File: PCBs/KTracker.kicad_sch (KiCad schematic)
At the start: 63 parts, among them J1 Conn_01x02_Female, J2 Conn_01x04_Female, J3 Conn_01x02_Female, J4 Conn_01x08_Female, J5 Conn_01x02_Female, P1 USB_C_Plug_USB2.0, SW1 Option/FLASH Switch, SW2 Cali Switch, SW3 SW_SPDT MAIN POWER, U1 ME6211C, U2 TP4056, U3 MPU-6050, U4 DW01, U5 FS8205A, U6 ESP-12F, U7 CH340C, U8 QMC5883L

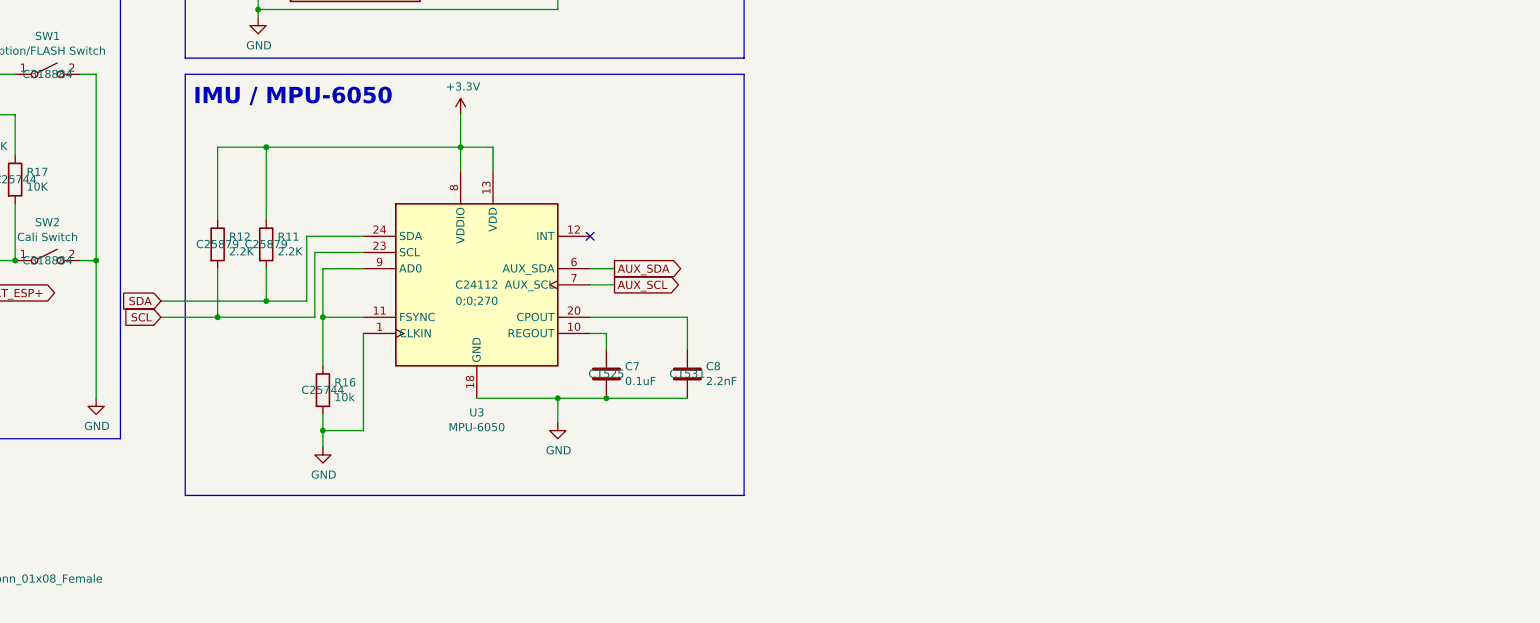
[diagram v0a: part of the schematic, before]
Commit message: #auto_saved_files#
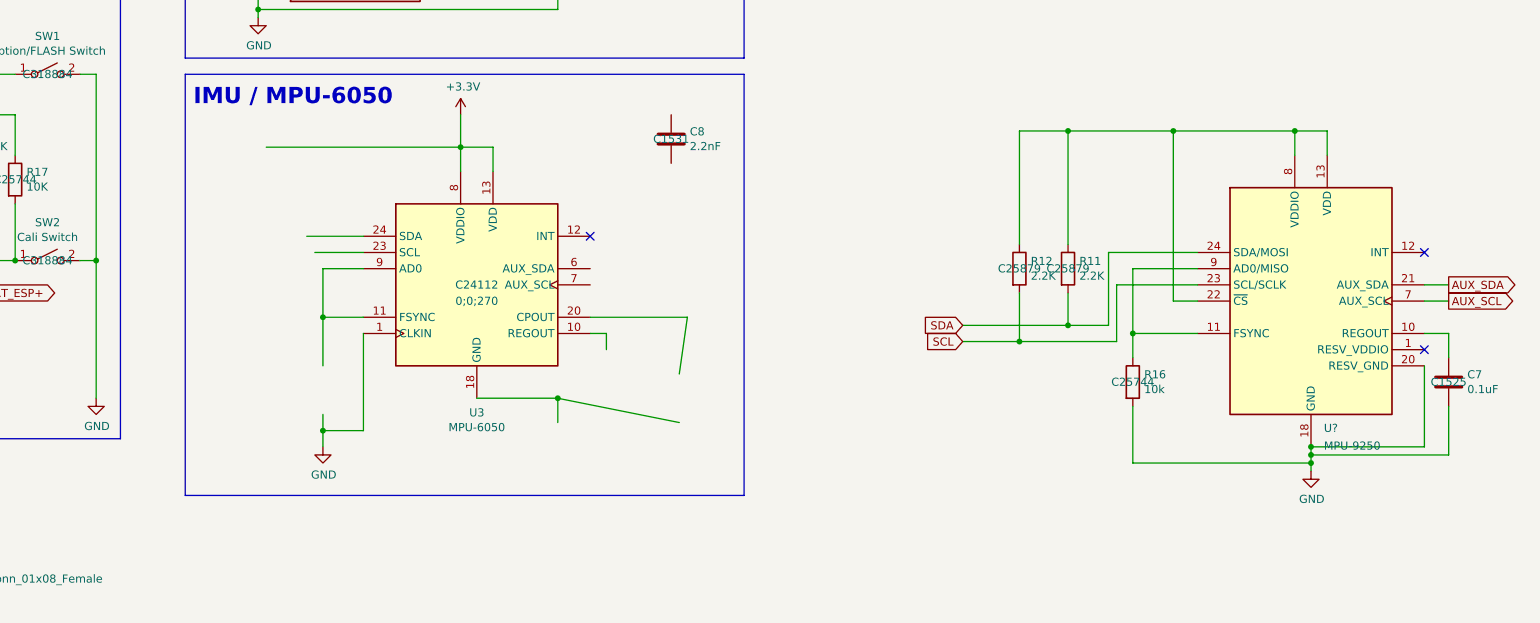
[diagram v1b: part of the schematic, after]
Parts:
- added U?: MPU-9250, Sensor_Motion:InvenSense_QFN-24_3x3mm_P0.4mm, symbol Sensor_Motion:MPU-9250
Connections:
- net +3V3: no longer R11.1, R12.1
- net AUX_SCL: now also U?.7 (AUX_SCL); no longer U3.7 (AUX_SCL)
- net AUX_SDA: now also U?.21 (AUX_SDA); no longer U3.6 (AUX_SDA)
- net GND: now also U?.18 (GND), U?.20 (RESV_GND); no longer C8.2, U3.18 (GND)
- net SCL: now also U?.23 (SCL/SCLK); no longer U3.23 (SCL)
- net SDA: now also U?.24 (SDA/MOSI); no longer U3.24 (SDA)
- net at U3.10 (REGOUT): no longer C7.1
- net at U3.11 (FSYNC), U3.9 (AD0): no longer R16.1
- net at U3.20 (CPOUT): no longer C8.1
- new net: R16.1, U?.11 (FSYNC), U?.9 (AD0/MISO)
- new net: C7.1, U?.10 (REGOUT)
- new net: R11.1, R12.1, U?.13 (VDD), U?.22 (~{CS}), U?.8 (VDDIO)
- no-connect marks 33 -> 35
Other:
- moved on the sheet: C7, C8, R11, R12, R16
